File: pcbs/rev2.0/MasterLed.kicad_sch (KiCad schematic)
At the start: 32 parts

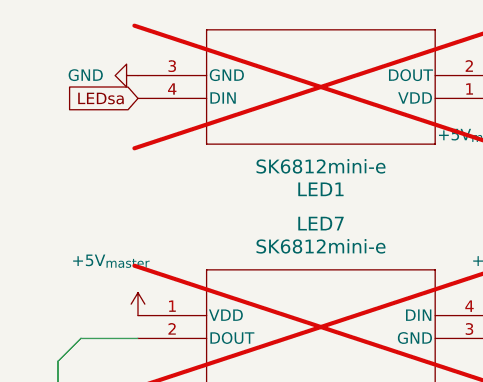
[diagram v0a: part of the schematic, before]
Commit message: start with leds
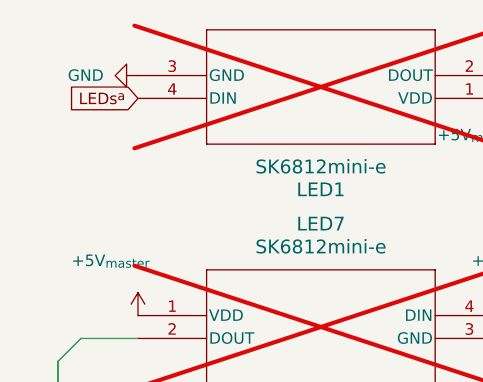
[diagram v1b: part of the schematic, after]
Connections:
- net LEDsa renamed LEDs^{a}
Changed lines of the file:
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@@
 		)
 	)
-	(global_label "LEDsa"
+	(global_label "LEDs^{a}"
 		(shape input)
 		(at 21.59 24.13 180)
@@
 		)
 		(property "Intersheetrefs" "${INTERSHEET_REFS}"
-			(at 12.9806 24.13 0)
+			(at 13.1596 24.13 0)
 			(effects
 				(font
